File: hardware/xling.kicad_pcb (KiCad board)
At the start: 2 copper layers, 37 x 59 mm, 63 parts, among them J2 TPS63031, J3 MCP73831, J4 USB_OTG, J5 AVR ISP, J6 Battery, Q1 TP0610T, SW1 Reset, SW2 Up, SW3 Select, SW4 Down, U1 SH1106G, U2 ATMEGA328P-AU, Y1 8MHz

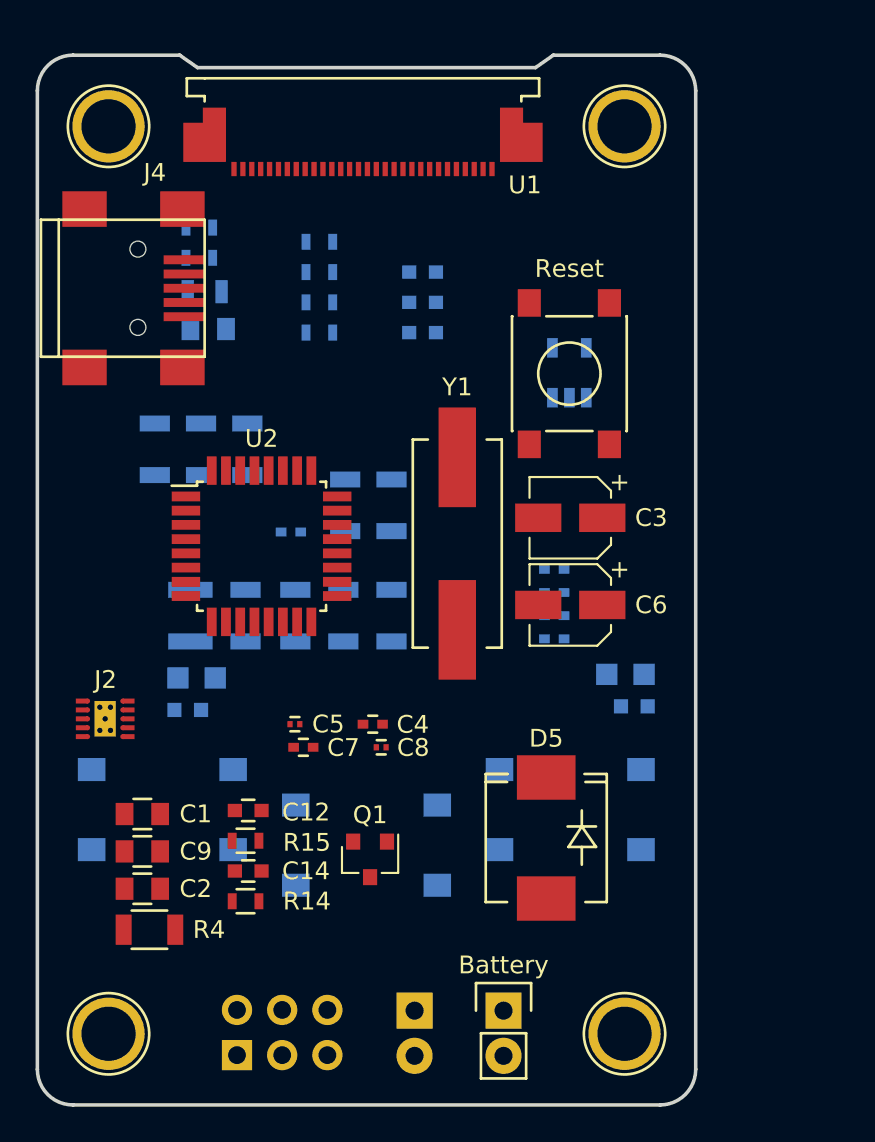
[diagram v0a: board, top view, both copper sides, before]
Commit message: patch 0.1.10: First PCB prototype.
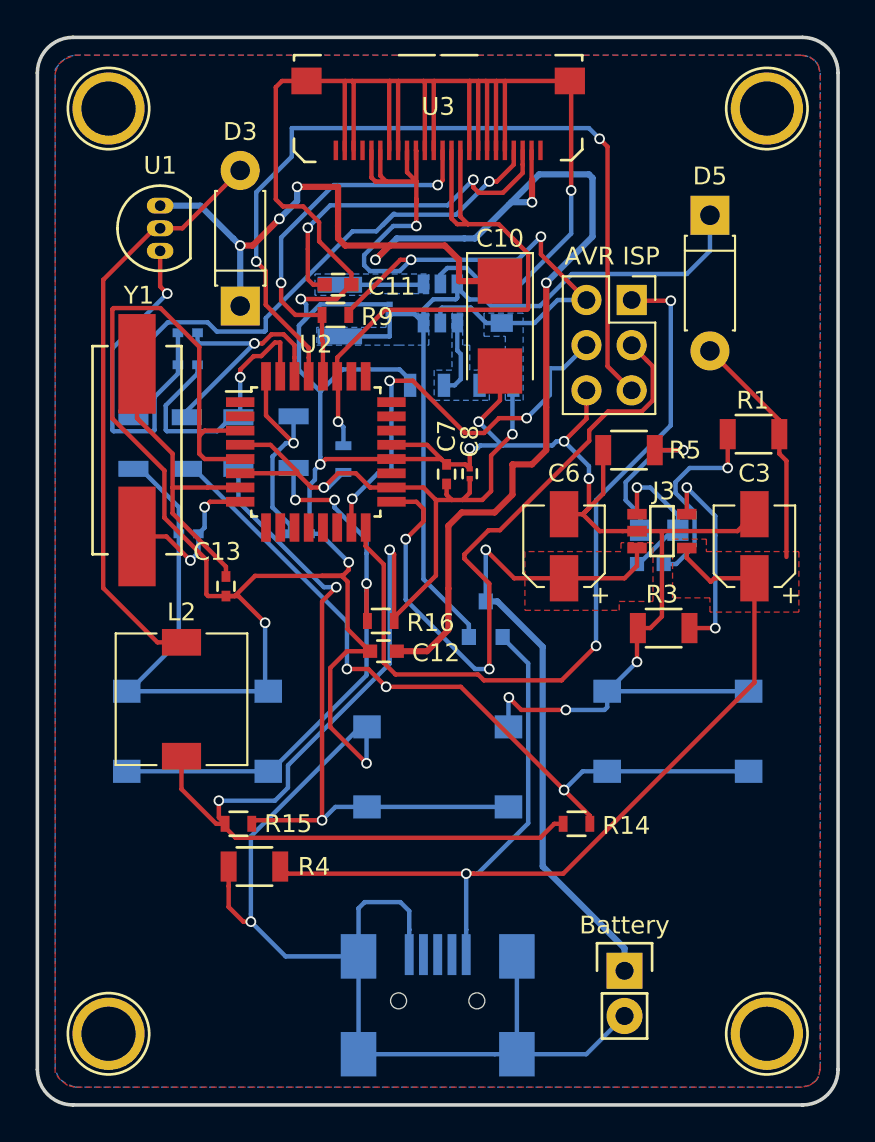
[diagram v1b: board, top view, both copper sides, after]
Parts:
- removed C14, C16: 2.2uF, Capacitors_SMD:C_0603
- removed C17, C2, C9: 10uF, Capacitors_SMD:C_0805
- removed C4: 10nF, Capacitors_SMD:C_0402
- removed D4: amber, LEDs:LED_0603
- removed J2: TPS63031, Xling Footprints:TPS63031_QFN_10
- removed JP1: D2D1, Pin_Headers:Pin_Header_Straight_1x02
- removed R10: 174K, Resistors_SMD:R_0805
- removed R11, R12, R13: 1K, Resistors_SMD:R_0603
- removed the REF** at (152.0, 134.0)
- removed the REF** at (123.0, 83.0)
- removed the REF** at (152.0, 83.0)
- removed SW1: Reset, Buttons_Switches_SMD:SW_SPST_PTS645
- added L2: 22uH, Inductors_SMD:L_7.3x7.3_H3.5, F.Cu at (127.1, 115.2)
- added REF**: 1pin, Connectors:1pin, F.Cu at (160.0, 134.0)
- added REF**: 1pin, Connectors:1pin, F.Cu at (160.0, 82.0)
- added REF**: 1pin, Connectors:1pin, F.Cu at (123.0, 82.0)
- added U3: DEP_128064I, Xling Footprints:XF2M_24151AR100_SMD_1x24_Pitch_0.5mm, F.Cu at (141.5, 81.2)
- added U4: MCP1640B-CH, TO_SOT_Packages_SMD:SOT-23-6, B.Cu at (141.7, 93.0)
- C1, J4, Q1: moved to B.Cu
- C10: value 2.2uF -> 33uF; footprint Capacitors_SMD:C_0603 -> Capacitors_Tantalum_SMD:CP_Tantalum_Case-C_EIA-6032-28_Reflow; moved to F.Cu
- C11, C13, J3, J5, R1, R16, R3, R5, R9: moved to F.Cu
- C5: value 0.1uF -> 4.7uF; moved to B.Cu
- D3: value green -> 1N5818; footprint LEDs:LED_0805 -> Diodes_THT:D_DO-41_SOD81_P7.62mm_Horizontal; moved to F.Cu
- D5: value B320 -> 1N5818; footprint Diodes_SMD:SMC_Standard -> Diodes_THT:D_DO-41_SOD81_P7.62mm_Horizontal
- L1: value 1.5uH -> 4.7uH
- R2: value 100K -> 910K
- R6: value 10K -> 191K; footprint Resistors_SMD:R_1206 -> Resistors_SMD:R_0805
- R7: value 10K -> 110K; footprint Resistors_SMD:R_1206 -> Resistors_SMD:R_0805
- U1: value SH1106G -> LT1109CZ-12; footprint Xling Footprints:Connector_FFC_FPC_MOLEX_524353071_30-pins -> TO_SOT_Packages_THT:TO-92_Inline_Narrow_Oval
- moved J5 47.9 mm to (152.4, 92.8), turned to 0 degrees
- moved J4 44.6 mm to (141.5, 133.0), turned to 90 degrees
- moved D5 36.2 mm to (156.8, 88.0)
- moved C1 35.0 mm to (145.1, 93.1), turned to 90 degrees
- moved R3 27.9 mm to (154.2, 111.2), turned to 180 degrees
- moved C18 26.0 mm to (127.5, 94.6)
- moved C19 24.3 mm to (127.5, 96.4)
- moved C5 23.9 mm to (138.8, 93.3), turned to 90 degrees
- moved R16 21.6 mm to (138.3, 110.8)
- moved C15 21.4 mm to (127.5, 105.9)
- moved D3 21.0 mm to (130.4, 93.1), turned to 90 degrees
- moved R1 20.7 mm to (159.2, 100.3), turned to 180 degrees
- moved R6 19.5 mm to (144.8, 97.6), turned to 180 degrees
- moved R14 19.1 mm to (149.3, 122.2)
- moved L1 19.1 mm to (136.0, 93.4)
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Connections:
- C10 pad 1: Net-(C10-Pad1) -> +12V
- C10 pad 2: Net-(C10-Pad2) -> GND
- C11 pad 2: Net-(C11-Pad2) -> GND
- C12 pad 1: +3V3 -> +12V
- D3 pad 1: Net-(D3-Pad1) -> +12V
- D5 pad 1: Net-(D5-Pad1) -> Net-(C5-Pad1)
- L1 pad 1: Net-(J2-Pad4) -> Net-(C5-Pad1)
- Q1 pad 2: Net-(D5-Pad1) -> Net-(C5-Pad1)
- R2 pad 1: Net-(C4-Pad1) -> GND
- R2 pad 2: Net-(D5-Pad1) -> Net-(R2-Pad2)
- R6 pad 2: /ISP_RST -> Net-(R6-Pad2)
- R7 pad 1: +3V3 -> Net-(R6-Pad2)
- U1 pad 2: Net-(C10-Pad1) -> Net-(D3-Pad2)
- U1 pad 3: Net-(C10-Pad2) -> +12V
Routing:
- net GND: track 0.00 -> 368.6 mm, vias 0 -> 15
- net +3V3: track 0.00 -> 134.9 mm, vias 0 -> 7
- net +12V: track 0.00 -> 84.2 mm, vias 0 -> 6
- net Net-(C3-Pad1): track 0.00 -> 75.7 mm, vias 0 -> 1
- net /ISP_RST: track 0.00 -> 48.4 mm, vias 0 -> 2
- net Net-(C5-Pad1): track 0.00 -> 46.7 mm
- net /ISP_PDO_MISO: track 0.00 -> 44.5 mm, vias 0 -> 2
- net Net-(R14-Pad2): track 0.00 -> 43.5 mm, vias 0 -> 3
- net /ISP_SCK: track 0.00 -> 38.9 mm, vias 0 -> 2
- net Net-(C6-Pad1): track 0.00 -> 37.7 mm, vias 0 -> 1
- net Net-(R15-Pad2): track 0.00 -> 37.6 mm, vias 0 -> 2
- net /OLED_SDA: track 0.00 -> 33.3 mm, vias 0 -> 1
- net Net-(D3-Pad2): track 0.00 -> 33.2 mm
- net Net-(R16-Pad2): track 0.00 -> 32.5 mm, vias 0 -> 3
- net Net-(R2-Pad2): track 0.00 -> 31.8 mm, vias 0 -> 1
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- added copper zone on B.Cu, net +3V3
- added copper zone on B.Cu, net GND
- added copper zone on F.Cu, net GND
- added copper zone on F.Cu, net Net-(C3-Pad1)
- added copper zone on B.Cu, net Net-(C5-Pad1)
- added copper zone on F.Cu, net Net-(C6-Pad1)
- added copper zone on B.Cu, net Net-(L1-Pad2)
- added copper zone on B.Cu, net Net-(R6-Pad2)
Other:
- board size 37 x 59 mm -> 45 x 60 mm
